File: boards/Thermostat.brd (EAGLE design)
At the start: 50.8 x 50.8 mm, 28 parts

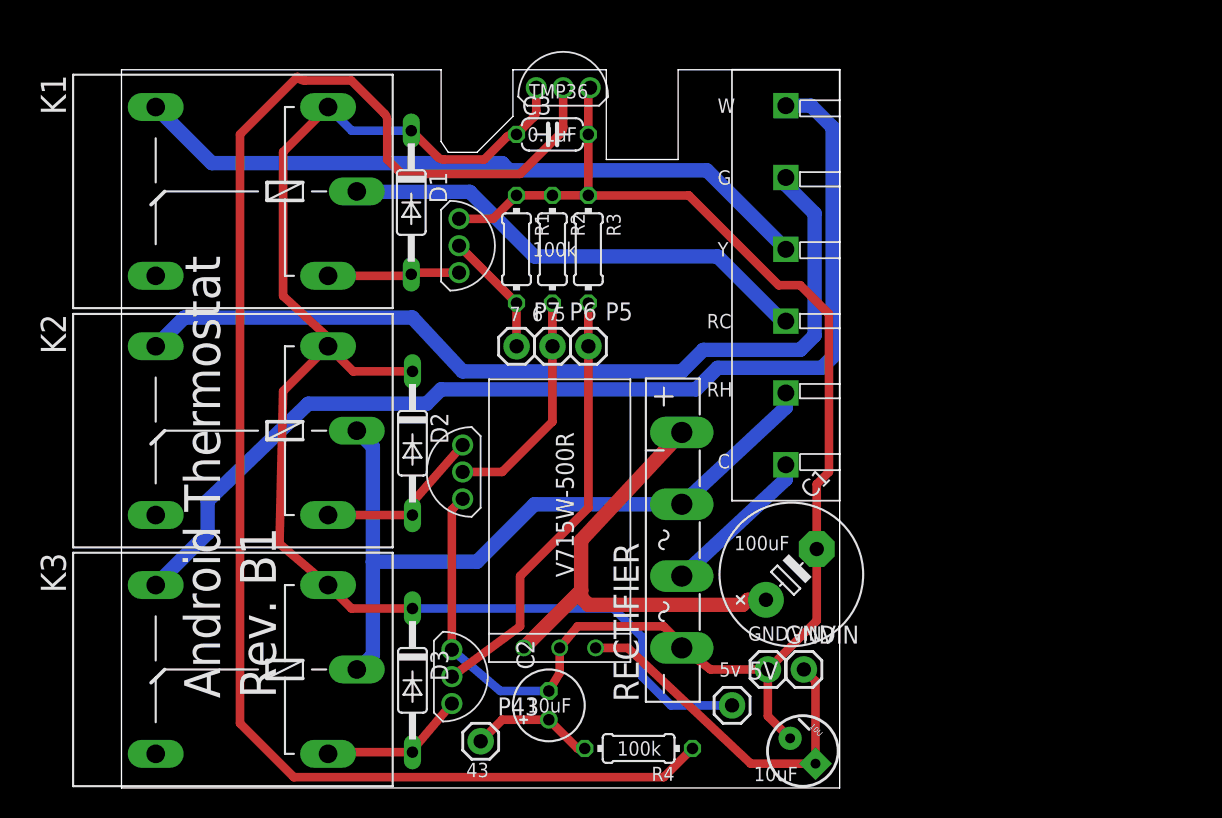
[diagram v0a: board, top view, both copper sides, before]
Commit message: put all the downloaded files into directories
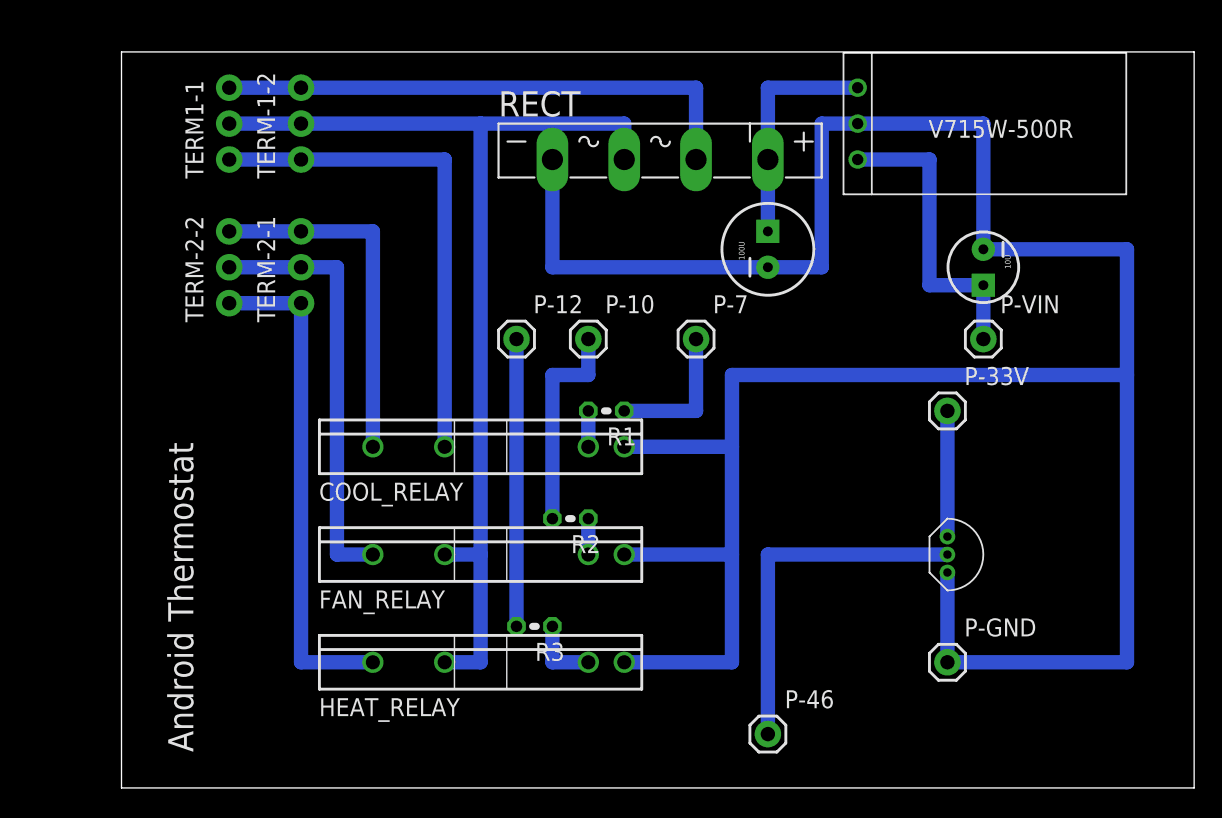
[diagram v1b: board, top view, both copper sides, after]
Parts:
- removed 5V, GND, P43, P5, P6, P7, VIN: (no value), SparkFun-Connectors:1X01
- removed C1: (no value), rcl:E5-10,5
- removed C2: (no value), rcl:E2-5
- removed C3: (no value), rcl:C050-024X044
- removed D1, D2, D3: (no value), diode:DO35-10
- removed K1, K2, K3: (no value), relay:G5LE
- removed R4: (no value), rcl:0204/7
- removed RECTIFIER: (no value), rectifier:GBU4S
- removed U$3: PHOENIX-651-1935200, android-thermostat:PHOENIX_E_5MM_6PIN
- removed U$4, U$5, U$6: TRANSISTOR, android-thermostat:TRANSISTOR
- added 100U: (no value), SparkFun-Passives:CPOL-RADIAL-100UF-25V
- added COOL_RELAY, FAN_RELAY, HEAT_RELAY: S101T01, relay:S102T0X
- added P-10, P-12, P-33V, P-46, P-7, P-GND, P-VIN: M01PTH, SparkFun-Connectors:1X01
- added RECT: (no value), rectifier:GBU4S
- added TERM-1-2, TERM-2-1, TERM-2-2, TERM1-1: (no value), SparkFun-Connectors:1X03_NO_SILK
- R1, R2, R3: device rcl:0204/7 -> resistor:0204V
- moved U$1 42.8 mm to (58.4, 16.5), turned to 0 degrees
- moved U$2 42.7 mm to (52.1, 47.0), turned to 0 degrees
- moved 10U 36.5 mm to (61.0, 36.8), turned to 270 degrees
- moved R3 26.9 mm to (29.2, 11.4), turned to 180 degrees
- moved R2 19.1 mm to (31.8, 19.1), turned to 180 degrees
- moved R1 13.1 mm to (34.3, 26.7), turned to 180 degrees
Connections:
- removed net +5V: 5V.1, C3.1, D1.C, D2.C, D3.C, K1.1, K2.1, K3.1, U$1.VC1
- removed net N$17: P5.1, R3.2, U$4.G
- removed net N$18: D3.A, K3.2, U$4.D
- removed net N$20: RECTIFIER.AC2, U$3.P$1
- removed net N$24: C1.+, RECTIFIER.+, U$2.VI
- new net N$11: P-33V.1, U$1.VCC-1
- new net N$12: 100U.1, RECT.+, U$2.VI
- new net N$8: P-12.1, R3.2
- new net P2: FAN_RELAY.2, HEAT_RELAY.2, RECT.AC2, TERM-1-2.2, TERM1-1.2
- net GND: now also 100U.2, COOL_RELAY.4, FAN_RELAY.4, HEAT_RELAY.4, P-GND.1, RECT.-, U$1.GND-3; no longer C1.-, C2.-, C3.2, GND.1, R1.1, R2.1, R3.1, RECTIFIER.-, U$1.GND3, U$4.S, U$5.S, U$6.S
- net N$1: now also COOL_RELAY.2, TERM-1-2.1, TERM1-1.1; no longer K1.P, U$3.P$3
- net N$10: now also P-VIN.1; no longer VIN.1
- net N$13: now also HEAT_RELAY.1, TERM-2-1.1, TERM-2-2.1; no longer K3.S, U$3.P$6
- net N$14: now also COOL_RELAY.1, TERM-2-1.3, TERM-2-2.3; no longer K1.S, U$3.P$4
- net N$15: now also FAN_RELAY.1, TERM-2-1.2, TERM-2-2.2; no longer K2.S, U$3.P$5
- net N$2: now also HEAT_RELAY.3, R3.1; no longer P6.1, R2.2, U$5.G
- net N$3: now also RECT.AC1, TERM-1-2.3, TERM1-1.3; no longer D2.A, K2.2, U$5.D
- net N$4: now also P-7.1, R1.1; no longer C2.+, P43.1, R4.2
- net N$5: now also P-46.1, U$1.DATA-2; no longer R4.1, U$1.OUT2
- net N$6: now also FAN_RELAY.3, R2.1; no longer P7.1, R1.2, U$6.G
- net N$7: now also P-10.1, R2.2; no longer D1.A, K1.2, U$6.D
- net N$9: now also COOL_RELAY.3, R1.2; no longer K2.P, K3.P, RECTIFIER.AC1, U$3.P$2
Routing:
- net +5V: track 99.6 -> 0.00 mm
- net N$5: track 109.4 -> 25.4 mm
- net GND: track 109.7 -> 186.7 mm
- net P2: track 0.00 -> 73.7 mm
- net N$9: track 52.5 -> 2.54 mm
- net N$13: track 76.0 -> 35.6 mm
- net N$24: track 33.7 -> 0.00 mm
- net N$15: track 62.2 -> 30.5 mm
- net N$17: track 30.9 -> 0.00 mm
- net N$3: track 12.3 -> 38.1 mm
- net N$14: track 49.0 -> 25.4 mm
- net N$8: track 0.00 -> 20.3 mm
- net N$12: track 0.00 -> 16.5 mm
- net N$2: track 16.2 -> 5.08 mm
- net N$20: track 11.1 -> 0.00 mm
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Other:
- board size 50.8 x 50.8 mm -> 75.9 x 52.1 mm
- board text removed: "0.1uF"
- board text removed: "100k"
- board text removed: "100uF"
- board text removed: "10uF"
- board text removed: "43"
- board text removed: "5v"
- board text removed: "7 6 5"
- board text removed: "C"
- board text removed: "G"
- board text removed: "GND"
- board text removed: "RC"
- board text removed: "RH"
- board text removed: "Rev B1"
- board text removed: "Rev. B1"
- board text removed: "TMP36"
- board text removed: "VIN"
- board text removed: "W"
- board text removed: "Y"
